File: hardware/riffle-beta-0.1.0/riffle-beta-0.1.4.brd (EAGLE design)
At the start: 104.8 x 18 mm, 50 parts, among them IC1 ATMEGA328P, IC3 CH340G, IC4 MCP1700-33, IC5 24AA128SN, IC6 MCP1700-33, J1 AYZ0202, U1 MCP73831T-2ACI/OT, X2 12MHz, X3 16 MHz

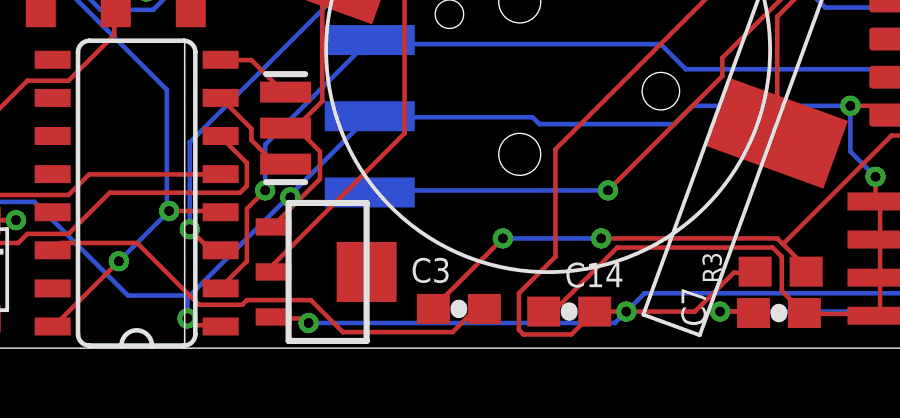
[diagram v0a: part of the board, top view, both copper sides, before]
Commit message: routed board
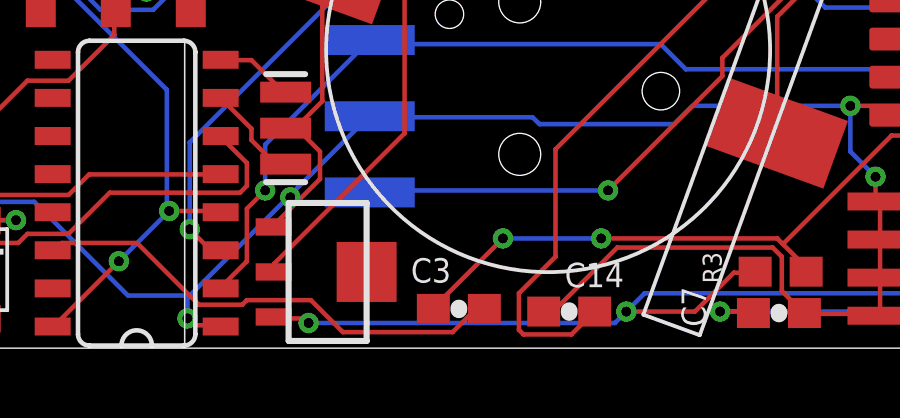
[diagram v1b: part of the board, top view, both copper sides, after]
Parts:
- renumbered CN1 to CNL
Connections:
- net VGEN1: now also D7.A, JP1.2; no longer CN2.1, D6.A
- net VGEN2: now also CN2.1, D6.A; no longer D7.A, JP1.2
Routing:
- net VGEN2: track 22.0 -> 24.6 mm, vias 4 -> 2
- net VGEN1: track 24.6 -> 22.0 mm, vias 2 -> 4
- net VCC: track 119.9 -> 118.7 mm
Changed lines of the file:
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@@
 </autorouter>
 <elements>
-<element name="CN1" library="adafruit" package="JST-PH-2-SMT-RA" value="" x="1.5906" y="4.6962" smashed="yes" rot="R90">
+<element name="CNL" library="adafruit" package="JST-PH-2-SMT-RA" value="" x="1.5906" y="4.6962" smashed="yes" rot="R90">
 <attribute name="VALUE" x="9.210609375" y="2.1562" size="1.27" layer="27" font="vector" rot="R90"/>
 </element>
@@
 <signals>
 <signal name="GND">
-<contactref element="CN1" pad="2"/>
+<contactref element="CNL" pad="2"/>
 <contactref element="IC1" pad="3"/>
 <contactref element="IC1" pad="5"/>
@@
 <contactref element="BATTPOWER" pad="2"/>
 <contactref element="JP5" pad="14"/>
-<contactref element="CN1" pad="1"/>
+<contactref element="CNL" pad="1"/>
 <contactref element="U1" pad="3"/>
 <contactref element="D5" pad="A"/>
@@
 <contactref element="R10" pad="2"/>
 <contactref element="C11" pad="2"/>
-<contactref element="IC4" pad="3"/>
-<contactref element="C14" pad="1"/>
 <wire x1="79.7052" y1="4.8006" x2="79.7052" y2="4.4196" width="0.1524" layer="1"/>
 <wire x1="79.4004" y1="5.1054" x2="79.7052" y2="4.8006" width="0.1524" layer="1"/>
@@
 <wire x1="53.0352" y1="15.3162" x2="53.0554" y2="15.3822" width="0.1524" layer="1"/>
 <wire x1="46.101" y1="1.2192" x2="43.815" y2="1.2192" width="0.1524" layer="1"/>
-<wire x1="43.815" y1="1.2192" x2="42.76" y2="1.2192" width="0.1524" layer="1"/>
 <wire x1="47.3964" y1="2.5146" x2="46.101" y2="1.2192" width="0.1524" layer="1"/>
 <wire x1="48.0822" y1="2.5146" x2="47.3964" y2="2.5146" width="0.1524" layer="1"/>
@@
 <wire x1="43.434" y1="0.8382" x2="33.2232" y2="0.8382" width="0.1524" layer="16"/>
 <wire x1="43.815" y1="1.2192" x2="43.434" y2="0.8382" width="0.1524" layer="16"/>
-<wire x1="32.0802" y1="0.9906" x2="32.0582" y2="1.04" width="0.1524" layer="1"/>
 <wire x1="48.9204" y1="14.097" x2="48.9204" y2="14.7066" width="0.1524" layer="1"/>
 <wire x1="41.4528" y1="6.6294" x2="48.9204" y2="14.097" width="0.1524" layer="1"/>
@@
 <wire x1="42.7482" y1="1.2192" x2="41.9862" y2="0.4572" width="0.1524" layer="1"/>
 <wire x1="48.9204" y1="14.7066" x2="48.9585" y2="14.7447" width="0.1524" layer="1"/>
-<wire x1="42.7482" y1="1.2192" x2="42.76" y2="1.2192" width="0.1524" layer="1"/>
 <wire x1="58.5978" y1="4.7244" x2="59.1312" y2="4.7244" width="0.1524" layer="16"/>
 <wire x1="55.7022" y1="1.8288" x2="58.5978" y2="4.7244" width="0.1524" layer="16"/>
@@
 <via x="64.9224" y="10.5156" extent="1-16" drill="0.3302"/>
 <via x="61.341" y="7.7724" extent="1-16" drill="0.3302"/>
+<contactref element="IC4" pad="3"/>
+<contactref element="C14" pad="1"/>
+<wire x1="42.7482" y1="1.2192" x2="42.76" y2="1.2192" width="0" layer="19" extent="1-1"/>
+<wire x1="43.434" y1="0.8382" x2="42.76" y2="1.2192" width="0" layer="19" extent="1-16"/>
+<wire x1="32.0582" y1="1.04" x2="32.0802" y2="0.9906" width="0" layer="19" extent="1-1"/>
 </signal>
 <signal name="AREF">
@@
 <wire x1="10.3144" y1="2.775" x2="10.3144" y2="2.775" width="0" layer="19" extent="1-16"/>
 </signal>
-<signal name="VGEN1">
+<signal name="VGEN2">
 <contactref element="CN2" pad="1"/>
 <contactref element="D6" pad="A"/>
@@
 <wire x1="15.4686" y1="16.8402" x2="15.4626" y2="16.8686" width="0.1524" layer="1"/>
 </signal>
-<signal name="VGEN2">
+<signal name="VGEN1">
 <contactref element="JP1" pad="2"/>
 <contactref element="D7" pad="A"/>

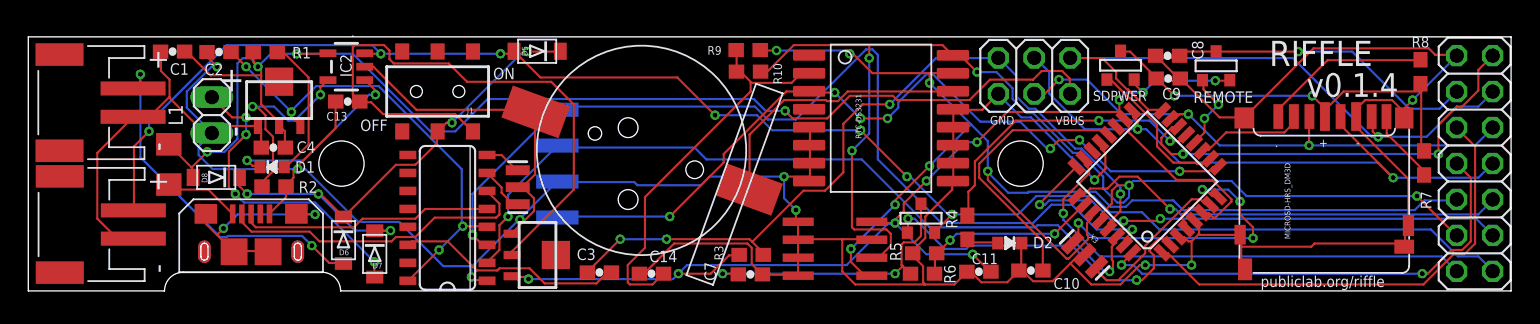
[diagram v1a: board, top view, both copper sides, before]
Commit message: update
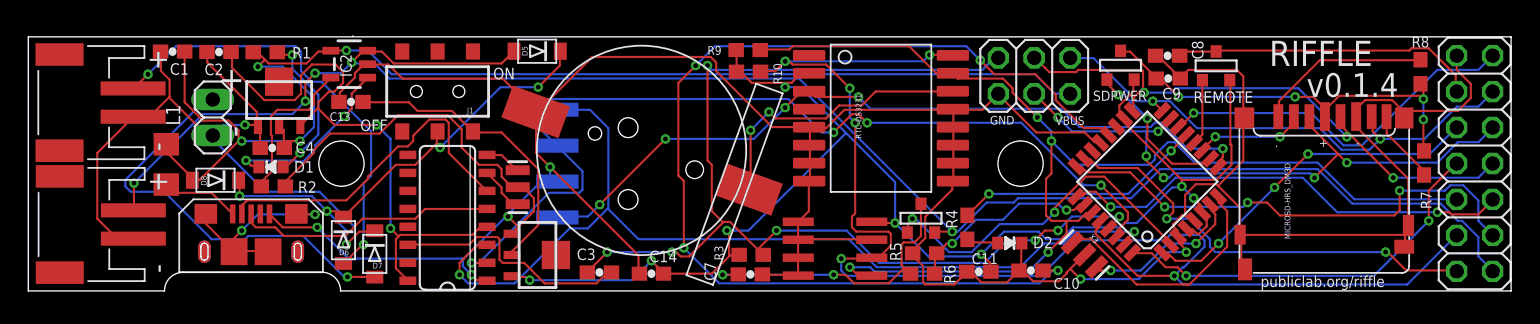
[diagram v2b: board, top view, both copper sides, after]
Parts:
- moved U1 0.27 mm to (20.5, 16.0)
- moved C13 0.23 mm to (20.7, 13.4)
- moved D8 0.21 mm to (11.1, 7.82)
- moved JP1 0.18 mm to (10.9, 12.3), turned to 270 degrees
- moved L1 0.18 mm to (7.62, 8.94)
- moved C4 0.08 mm to (15.1, 10.1)
- moved D1 0.08 mm to (15.0, 8.76)
- moved R2 0.05 mm to (15.2, 7.39)
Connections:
- net GND: now also JP1.2; no longer JP1.1
- net VGEN1: now also JP1.1; no longer JP1.2
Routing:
- net AREF: track 19.7 -> 75.0 mm, vias 0 -> 4
- net RESET: track 55.3 -> 77.8 mm, vias 4 -> 7
- net GND: track 286.9 -> 309.1 mm, vias 10 -> 7
- net N$1: track 43.1 -> 21.2 mm
- net SCL: track 80.9 -> 98.2 mm, vias 5 -> 6
- net VCC: track 118.7 -> 104.2 mm, vias 9 -> 8
- net VBAT: track 114.7 -> 126.8 mm, vias 7 -> 5
- net RXD: track 56.0 -> 67.4 mm, vias 2 -> 4
- net D3: track 33.0 -> 25.0 mm, vias 0 -> 3
- net VGEN1: track 22.0 -> 29.5 mm, vias 4 -> 1
- net VGEN2: track 24.6 -> 31.5 mm
- net N$8: track 33.8 -> 40.5 mm, vias 4 -> 2
- net MISO: track 43.5 -> 37.1 mm, vias 1 -> 2
- net MOSI: track 38.7 -> 43.9 mm, vias 3 -> 6
- net D2: track 33.0 -> 28.1 mm
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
